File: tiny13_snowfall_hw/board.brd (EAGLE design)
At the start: 20 x 19 mm, 6 parts, among them IC1 TINY13V-10SSU, X1 SSW-103-02-G-D, X2 SSW-104-02-G-S, X3 SSW-104-02-G-S

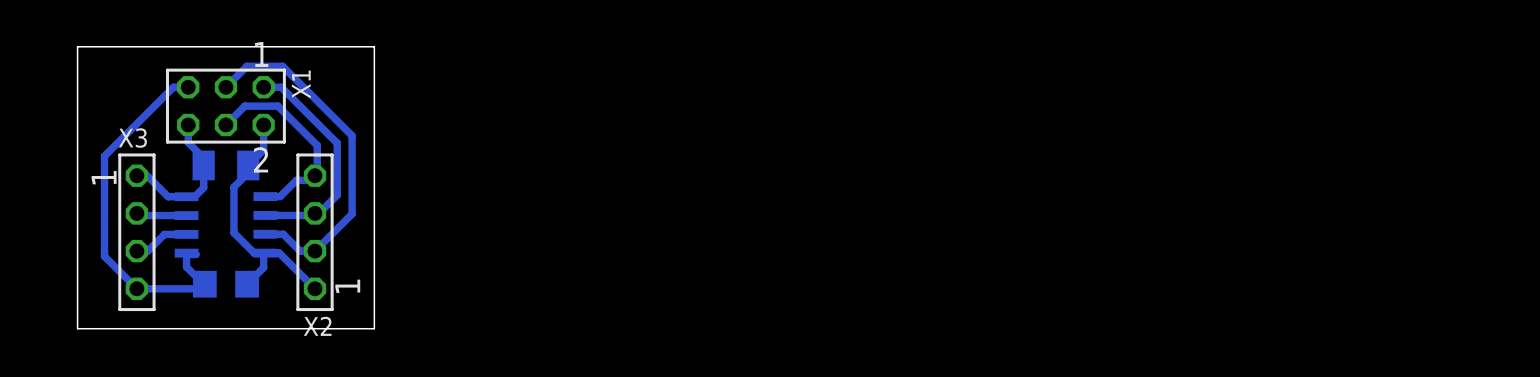
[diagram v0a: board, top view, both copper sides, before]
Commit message: optimized snowfall hw
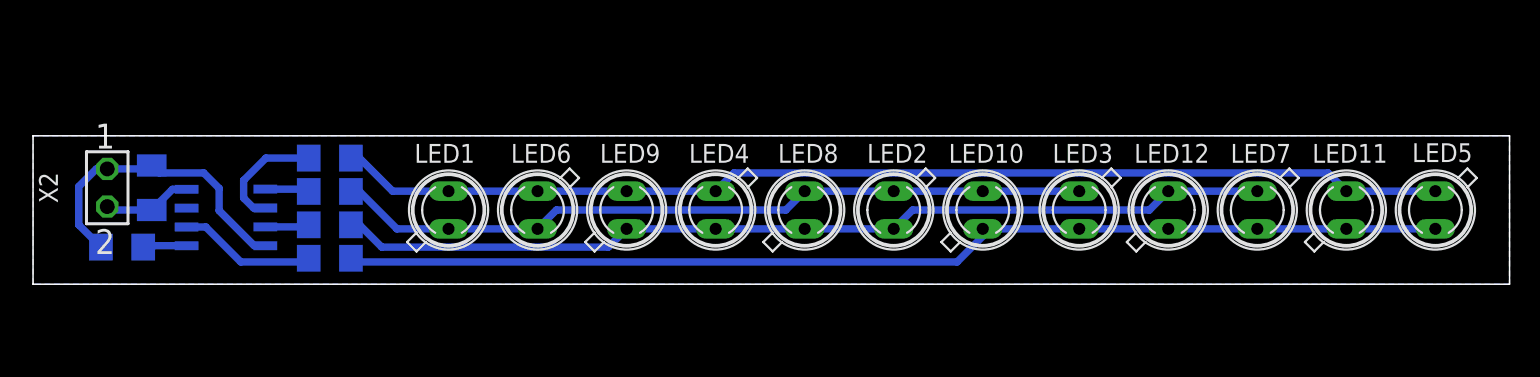
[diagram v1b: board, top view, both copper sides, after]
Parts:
- removed X1: SSW-103-02-G-D, con-samtec:SSW-103-02-G-D
- removed X3: SSW-104-02-G-S, con-samtec:SSW-104-02-G-S
- added LED1, LED10, LED11, LED12, LED2, LED3, LED4, LED5, LED6, LED7, LED8, LED9: (no value), led:SFH480
- added R2, R3, R4: 150R, rcl:R1206
- added R5: 10k, rcl:R1206
- IC1: value TINY13V-10SSU -> TINY13V
- R1: value 10k -> 150R
- X2: value SSW-104-02-G-S -> PWR; device con-samtec:SSW-104-02-G-S -> con-samtec:SSW-101-02-G-D
- moved X2 14.3 mm to (10.0, 24.5), turned to 180 degrees
- moved R1 9.38 mm to (25.0, 24.2)
- moved C1 5.22 mm to (13.0, 24.5), turned to 270 degrees
- moved IC1 0.50 mm to (18.0, 22.5)
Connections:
- removed net N$1: IC1.3, X3.2
- removed net N$2: IC1.2, X3.3
- removed net SCK: IC1.7, X1.3, X2.2
- removed net SI: IC1.5, X1.4, X2.4
- removed net SO: IC1.6, X1.1, X2.3
- new net PB0/SI: IC1.5, R1.1
- new net PB1/SO: IC1.6, R2.1
- new net PB2SCK: IC1.7, R3.1
- new net PB3: IC1.2, R4.1
- new net SIG0: LED1.K, LED10.A, LED2.K, LED3.K, LED6.A, LED8.A, R1.2
- new net SIG1: LED1.A, LED11.A, LED4.K, LED5.K, LED6.K, LED9.A, R2.2
- new net SIG2: LED12.A, LED2.A, LED4.A, LED7.K, LED8.K, LED9.K, R3.2
- new net SIG3: LED10.K, LED11.K, LED12.K, LED3.A, LED5.A, LED7.A, R4.2
- net GND: now also X2.2; no longer X1.6, X3.1
- net RST: now also R5.1; no longer R1.1, X1.5, X3.4
- net VCC: now also R5.2; no longer R1.2, X1.2
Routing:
- net SIG3: track 0.00 -> 75.1 mm
- net SIG1: track 0.00 -> 75.0 mm
- net SIG2: track 0.00 -> 63.3 mm
- net SIG0: track 0.00 -> 51.2 mm
- net SCK: track 23.6 -> 0.00 mm
- net RST: track 25.4 -> 2.96 mm
- net SO: track 16.0 -> 0.00 mm
- net SI: track 13.8 -> 0.00 mm
- net PB3: track 0.00 -> 9.31 mm
- net PB1/SO: track 0.00 -> 7.94 mm
- net GND: track 10.2 -> 6.25 mm
- net N$2: track 3.81 -> 0.00 mm
- net N$1: track 3.41 -> 0.00 mm
- net VCC: track 18.2 -> 21.2 mm
- net PB0/SI: track 0.00 -> 2.99 mm
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- added copper zone on layer 16, net GND
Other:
- board size 20 x 19 mm -> 99.5 x 10 mm
